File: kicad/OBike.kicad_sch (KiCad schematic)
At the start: 62 parts, among them J1 62684-402100ALF, J2 Micro_SD_Card_Det1, J3 Conn_01x02, J5 U.FL-R-SMT-1_10_, J6 Conn_01x02, SW1 5_position_tactile, U1 DPS368XTSA1, U10 MAX40200AUK, U2 DS3231M, U3 MCP23017_SO, U4 74HC14, U5 Seeed Studio XIAO SAMD21, U6 MAX40200AUK, U7 LC76G, U8 MAX40200AUK, U9 W25N01GVZEIG_TR

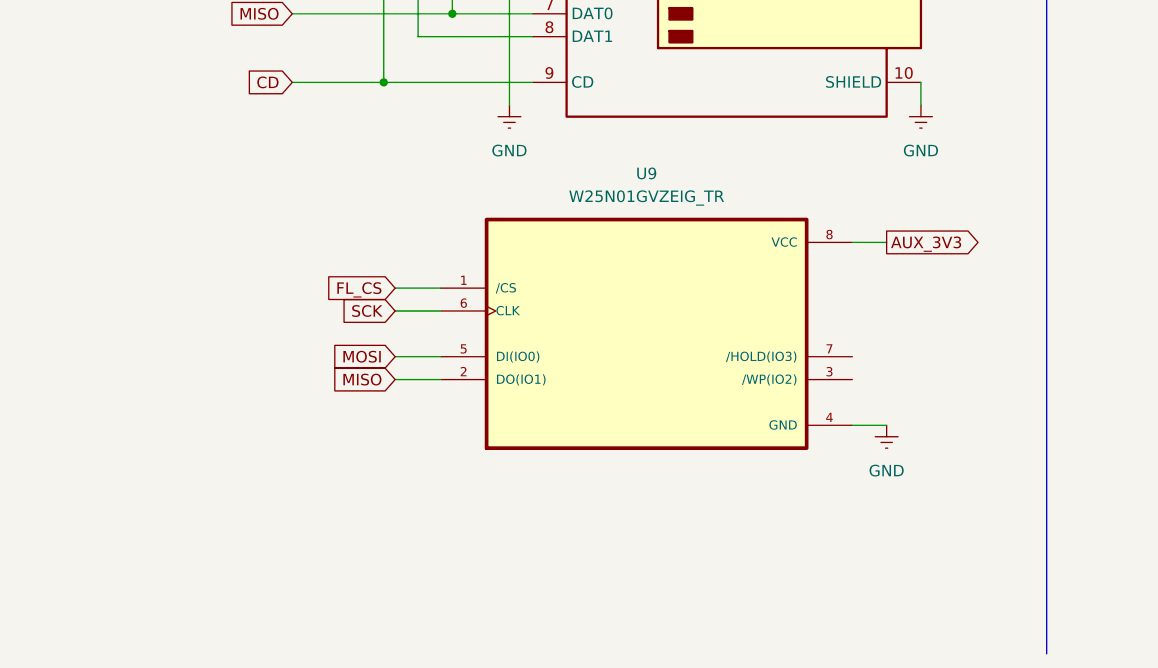
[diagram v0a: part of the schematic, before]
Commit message: Purchased PCBs
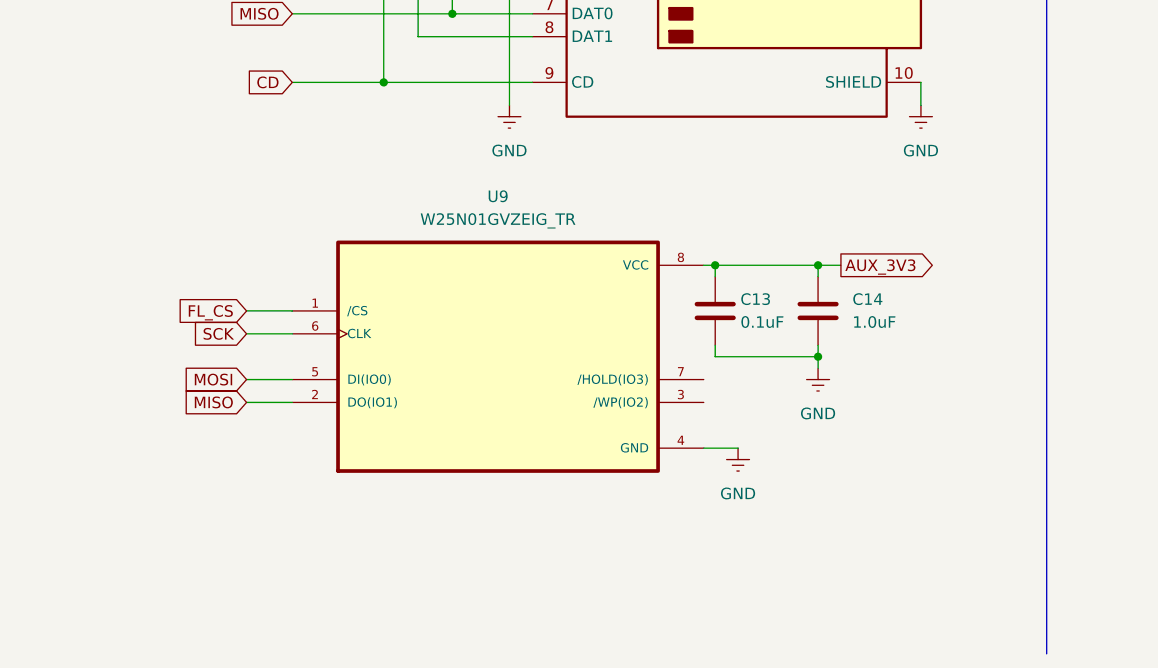
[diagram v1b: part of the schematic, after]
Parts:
- added C13: 0.1uF, Capacitor_SMD:C_0805_2012Metric, symbol Device:C
- added C14: 1.0uF, Capacitor_SMD:C_0805_2012Metric, symbol Device:C
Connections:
- net AUX_3V3: now also C13.1, C14.1
- net GND: now also C13.2, C14.2
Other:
- moved on the sheet: U9
